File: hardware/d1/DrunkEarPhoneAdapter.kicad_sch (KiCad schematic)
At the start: 0 parts

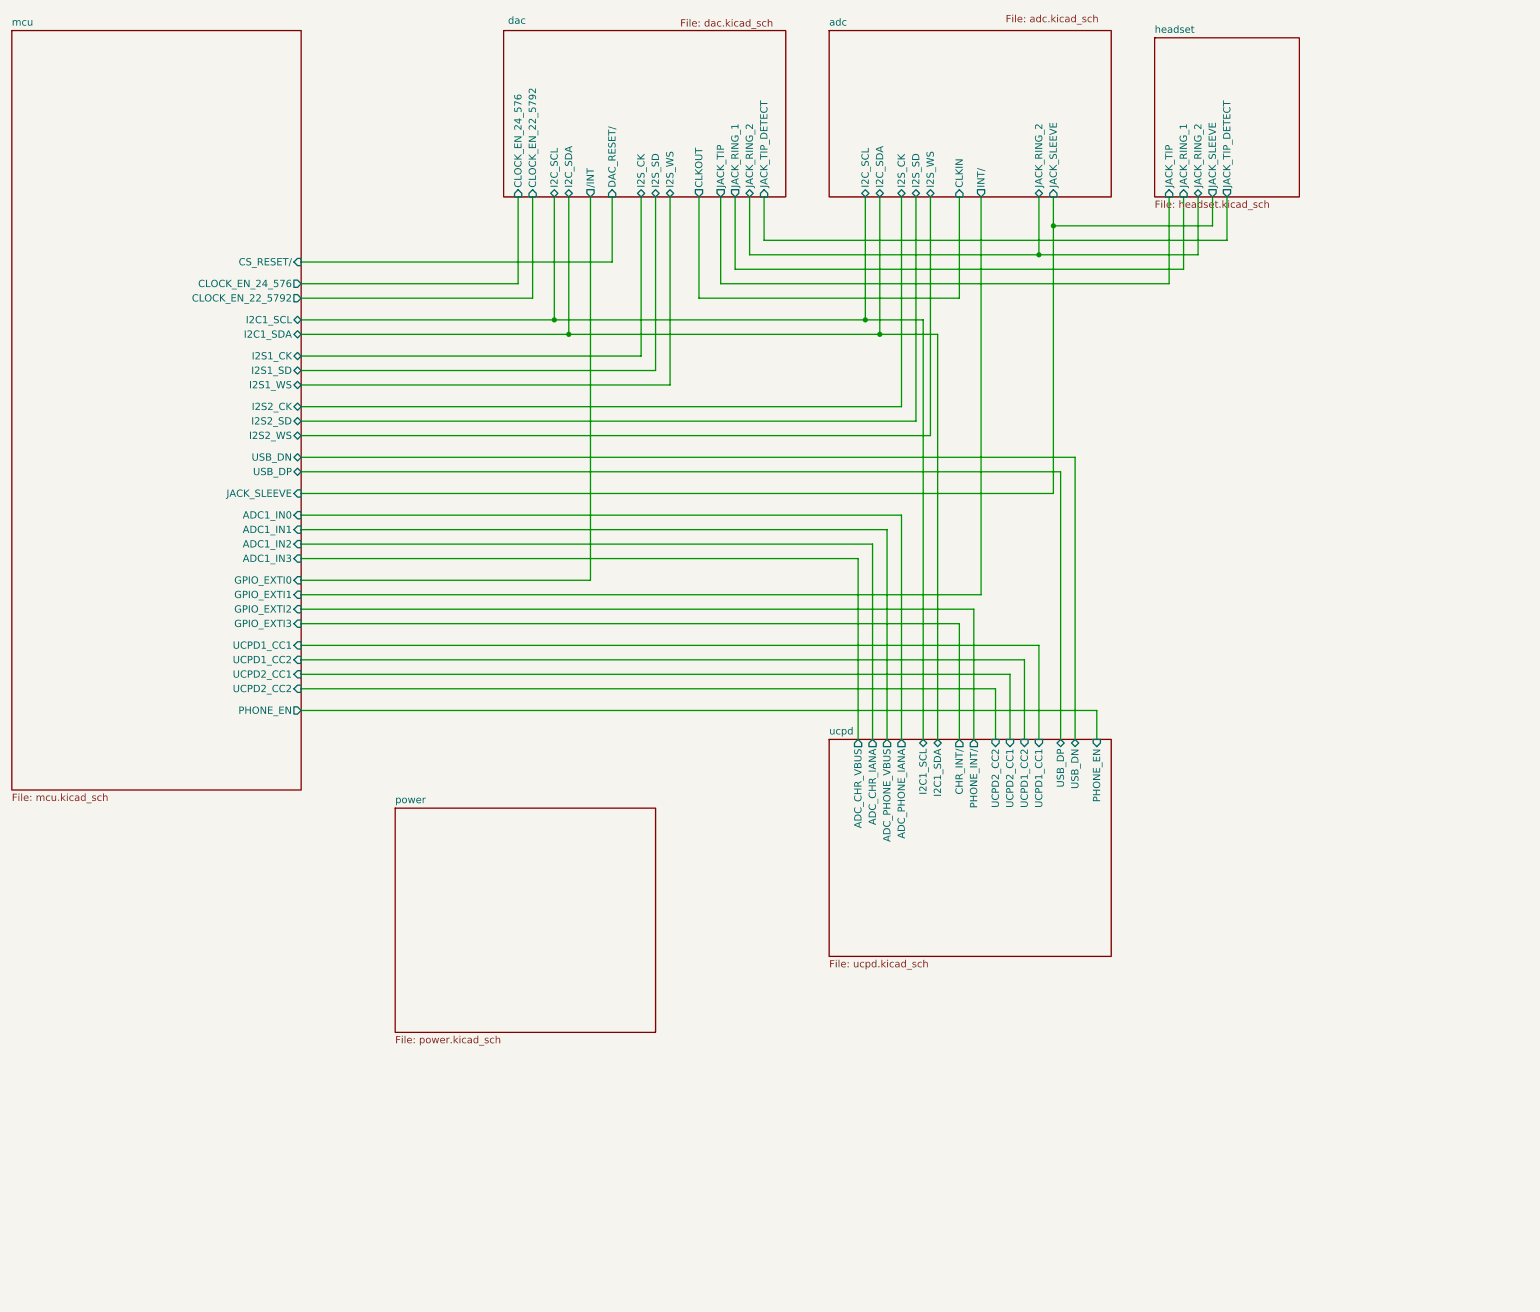
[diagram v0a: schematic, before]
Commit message: Fixes
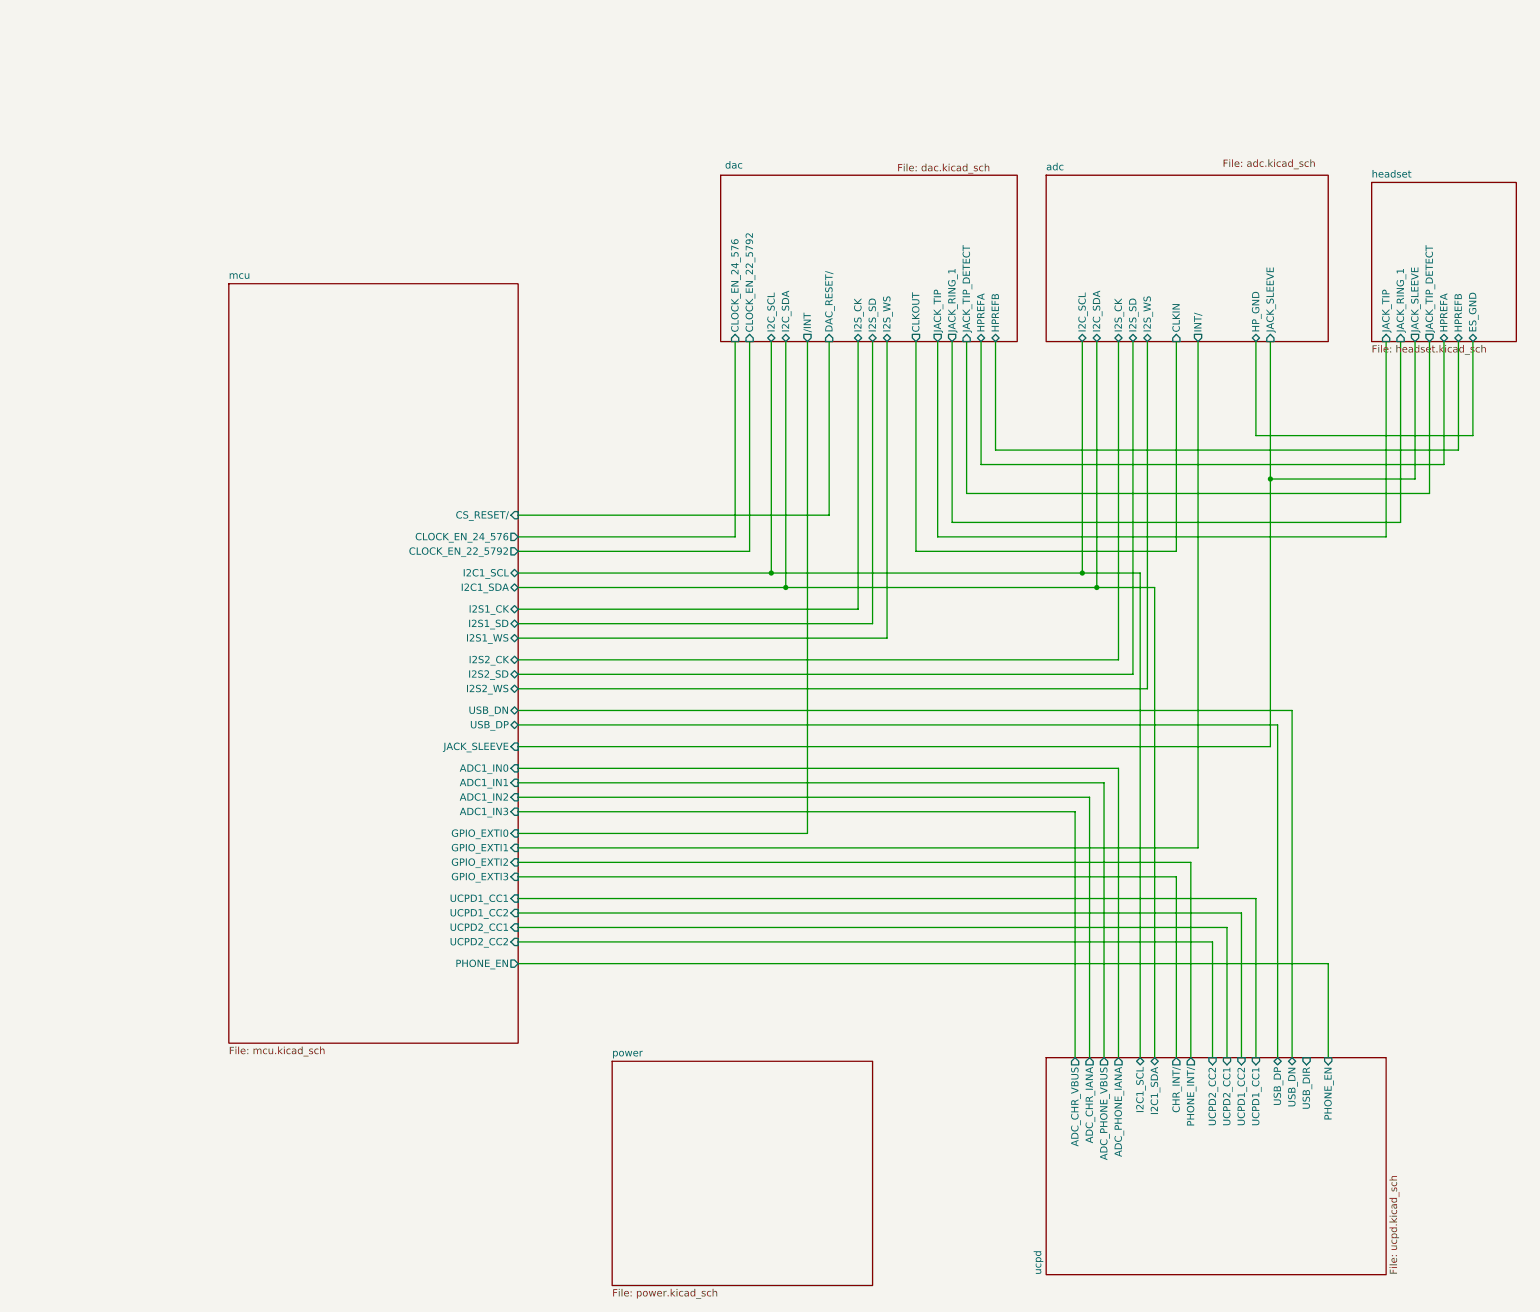
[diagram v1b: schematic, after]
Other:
- sheet adc ports: added HP_GND; removed JACK_RING_2
- sheet dac ports: added HPREFA, HPREFB; removed JACK_RING_2
- sheet headset ports: added ES_GND, HPREFA, HPREFB; removed JACK_RING_2
- sheet ucpd ports: added USB_DIR; removed none
